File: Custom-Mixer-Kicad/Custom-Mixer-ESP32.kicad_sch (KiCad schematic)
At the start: 39 parts, among them J1 Conn_01x08, SW1 RotaryEncoder_Switch, SW10 SW_Push, SW11 SW_Push, SW12 SW_Push, SW13 SW_Push, SW14 SW_Push, SW15 SW_Push, SW16 SW_Push, SW17 SW_Push, SW18 SW_Push, SW19 SW_Push, SW2 RotaryEncoder_Switch, SW21 SW_Push, SW3 SW_Push, SW4 SW_Push, SW5 SW_Push, SW6 SW_Push, SW7 SW_Push, SW8 SW_Push, SW9 SW_Push, U7 ESP32-S3-DevKitC, U8 MCP23017_SP

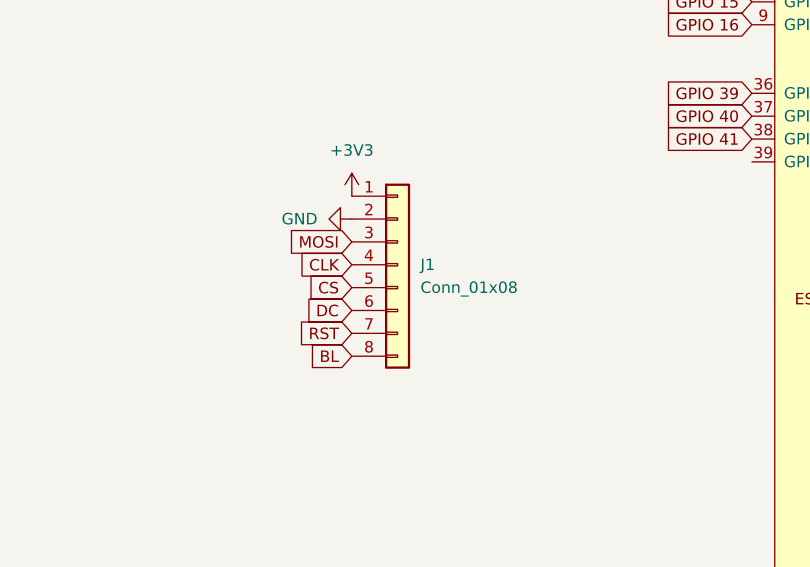
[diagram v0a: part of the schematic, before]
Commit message: PCB rework completed
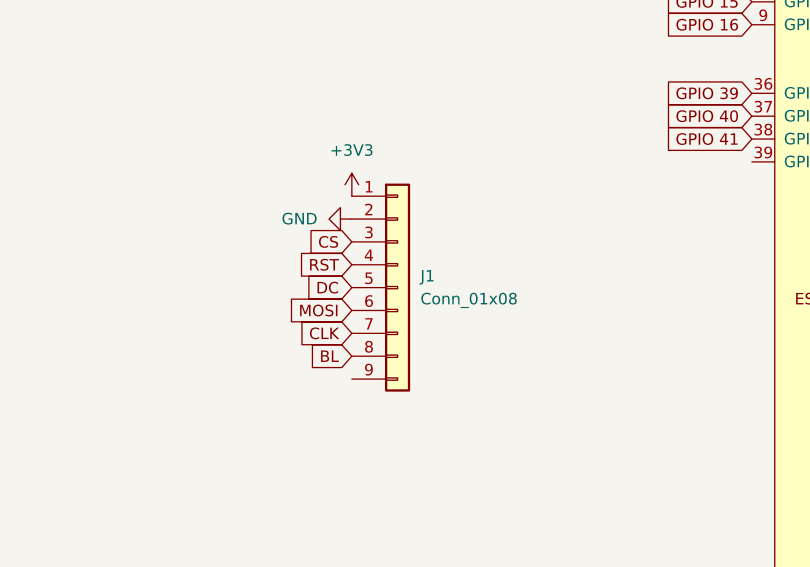
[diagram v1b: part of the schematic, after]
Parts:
- J1: footprint Connector_PinHeader_2.54mm:PinHeader_1x08_P2.54mm_Vertical -> Connector_PinSocket_2.54mm:PinSocket_1x09_P2.54mm_Vertical; symbol Connector_Generic:Conn_01x08 -> Connector_Generic:Conn_01x09
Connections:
- net CLK: now also J1.7 (Pin_7); no longer J1.4 (Pin_4)
- net CS: now also J1.3 (Pin_3); no longer J1.5 (Pin_5)
- net DC: now also J1.5 (Pin_5); no longer J1.6 (Pin_6)
- net MOSI: now also J1.6 (Pin_6); no longer J1.3 (Pin_3)
- net RST: now also J1.4 (Pin_4); no longer J1.7 (Pin_7)
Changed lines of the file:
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@@
 	(global_label "RST"
 		(shape input)
-		(at 95.25 85.09 180)
+		(at 95.25 77.47 180)
 		(fields_autoplaced yes)
 		(effects
@@
 		)
 		(property "Intersheetrefs" "${INTERSHEET_REFS}"
-			(at 88.8177 85.09 0)
+			(at 88.8177 77.47 0)
 			(effects
 				(font
@@
 	(global_label "CS"
 		(shape input)
-		(at 95.25 80.01 180)
+		(at 95.25 74.93 180)
 		(fields_autoplaced yes)
 		(effects
@@
 		)
 		(property "Intersheetrefs" "${INTERSHEET_REFS}"
-			(at 89.7853 80.01 0)
+			(at 89.7853 74.93 0)
 			(effects
 				(font
@@
 	(global_label "CLK"
 		(shape input)
-		(at 95.25 77.47 180)
+		(at 95.25 85.09 180)
 		(fields_autoplaced yes)
 		(effects
@@
 		)
 		(property "Intersheetrefs" "${INTERSHEET_REFS}"
-			(at 88.6967 77.47 0)
+			(at 88.6967 85.09 0)
 			(effects
 				(font
@@
 	(global_label "DC"
 		(shape input)
-		(at 95.25 82.55 180)
+		(at 95.25 80.01 180)
 		(fields_autoplaced yes)
 		(effects
@@
 		)
 		(property "Intersheetrefs" "${INTERSHEET_REFS}"
-			(at 89.7248 82.55 0)
+			(at 89.7248 80.01 0)
 			(effects
 				(font
@@
 	(global_label "MOSI"
 		(shape input)
-		(at 95.25 74.93 180)
+		(at 95.25 82.55 180)
 		(fields_autoplaced yes)
 		(effects
@@
 		)
 		(property "Intersheetrefs" "${INTERSHEET_REFS}"
-			(at 87.6686 74.93 0)
+			(at 87.6686 82.55 0)
 			(effects
 				(font
@@
 	)
 	(symbol
-		(lib_id "Connector_Generic:Conn_01x08")
-		(at 100.33 77.47 0)
+		(lib_id "Connector_Generic:Conn_01x09")
+		(at 100.33 80.01 0)
 		(unit 1)
 		(exclude_from_sim no)
@@
 		(fields_autoplaced yes)
 		(property "Reference" "J1"
-			(at 102.87 77.4699 0)
+			(at 102.87 78.7399 0)
 			(effects
 				(font
@@
 		)
 		(property "Value" "Conn_01x08"
-			(at 102.87 80.0099 0)
+			(at 102.87 81.2799 0)
 			(effects
 				(font
@@
 			)
 		)
-		(property "Footprint" "Connector_PinHeader_2.54mm:PinHeader_1x08_P2.54mm_Vertical"
-			(at 100.33 77.47 0)
+		(property "Footprint" "Connector_PinSocket_2.54mm:PinSocket_1x09_P2.54mm_Vertical"
+			(at 100.33 80.01 0)
 			(effects
 				(font
@@
 		)
 		(property "Datasheet" "~"
-			(at 100.33 77.47 0)
+			(at 100.33 80.01 0)
 			(effects
 				(font
@@
 			)
 		)
-		(property "Description" "Generic connector, single row, 01x08, script generated (kicad-library-utils/schlib/autogen/connector/)"
-			(at 100.33 77.47 0)
+		(property "Description" "Generic connector, single row, 01x09, script generated (kicad-library-utils/schlib/autogen/connector/)"
+			(at 100.33 80.01 0)
 			(effects
 				(font
@@
 		(pin "1"
 		)
+		(pin "9"
+		)
 		(instances
